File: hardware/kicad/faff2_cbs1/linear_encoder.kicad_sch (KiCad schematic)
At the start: 22 parts, among them J601 FH12-10S-0.5SH(55), J602 FTSH-105-01-L-DV-K-TR, J603 8510-4500PL, U601 AM26LV32

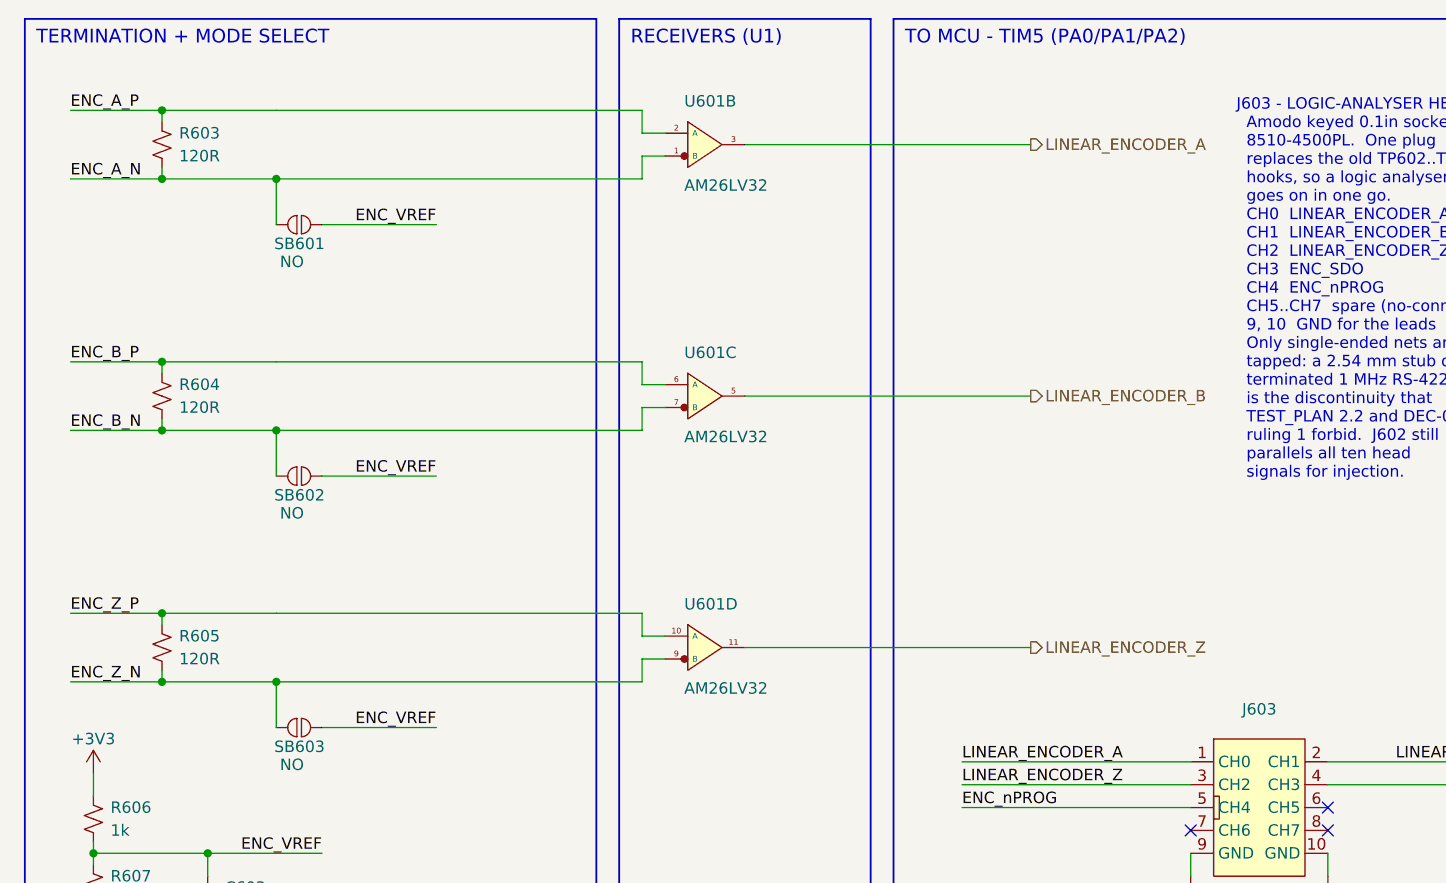
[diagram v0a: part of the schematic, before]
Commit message: Hand tweaks by human
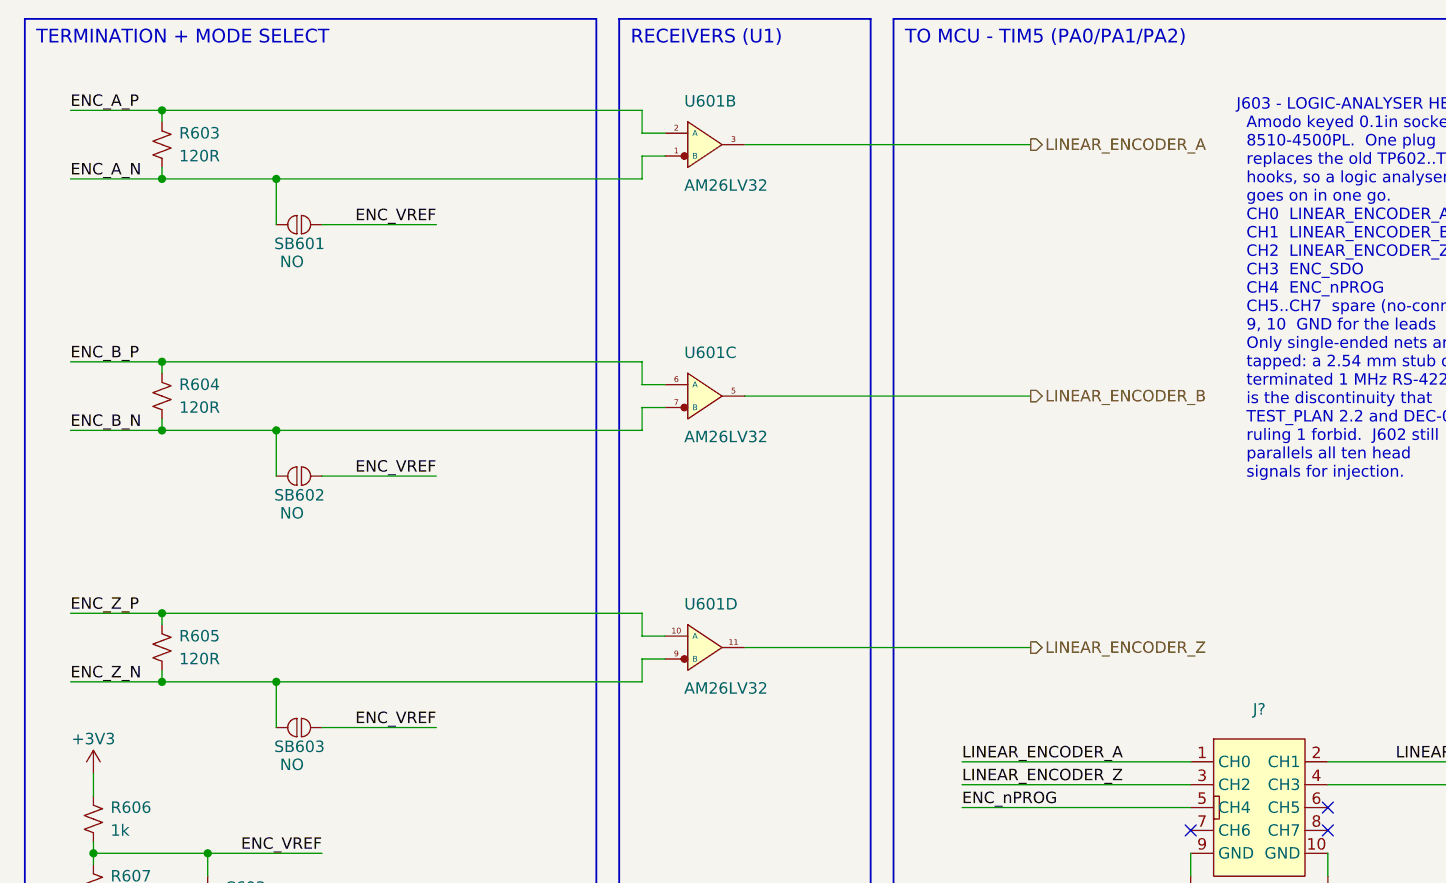
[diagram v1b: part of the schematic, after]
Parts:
- renumbered J603 to J?
